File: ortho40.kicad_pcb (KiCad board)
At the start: 2 copper layers, 229 x 79.3 mm, 120 parts, among them J1 USB_mini_micro_B, K11 KEYSW, K110 KEYSW, K111 KEYSW, K112 KEYSW, K12 KEYSW, K13 KEYSW, K14 KEYSW, K15 KEYSW, K16 KEYSW, K17 KEYSW, K18 KEYSW, K19 KEYSW, K21 KEYSW, K210 KEYSW, K211 KEYSW, K212 KEYSW, K22 KEYSW, K23 KEYSW, K24 KEYSW, K25 KEYSW, K26 KEYSW, K27 KEYSW, K28 KEYSW, K29 KEYSW, K2U1 KEYSW, K2U2 KEYSW, K2U3 KEYSW, K31 KEYSW, K310 KEYSW, K311 KEYSW, K312 KEYSW, K32 KEYSW, K33 KEYSW, K34 KEYSW, K35 KEYSW, K36 KEYSW, K37 KEYSW, K38 KEYSW, K39 KEYSW, K41 KEYSW, K410 KEYSW, K411 KEYSW, K412 KEYSW, K42 KEYSW, K43 KEYSW, K44 KEYSW, K45 KEYSW, K46 KEYSW, K47 KEYSW, K48 KEYSW, K49 KEYSW, SW1 SW_PUSH, U1 ATMEGA32U4, X1 XTAL

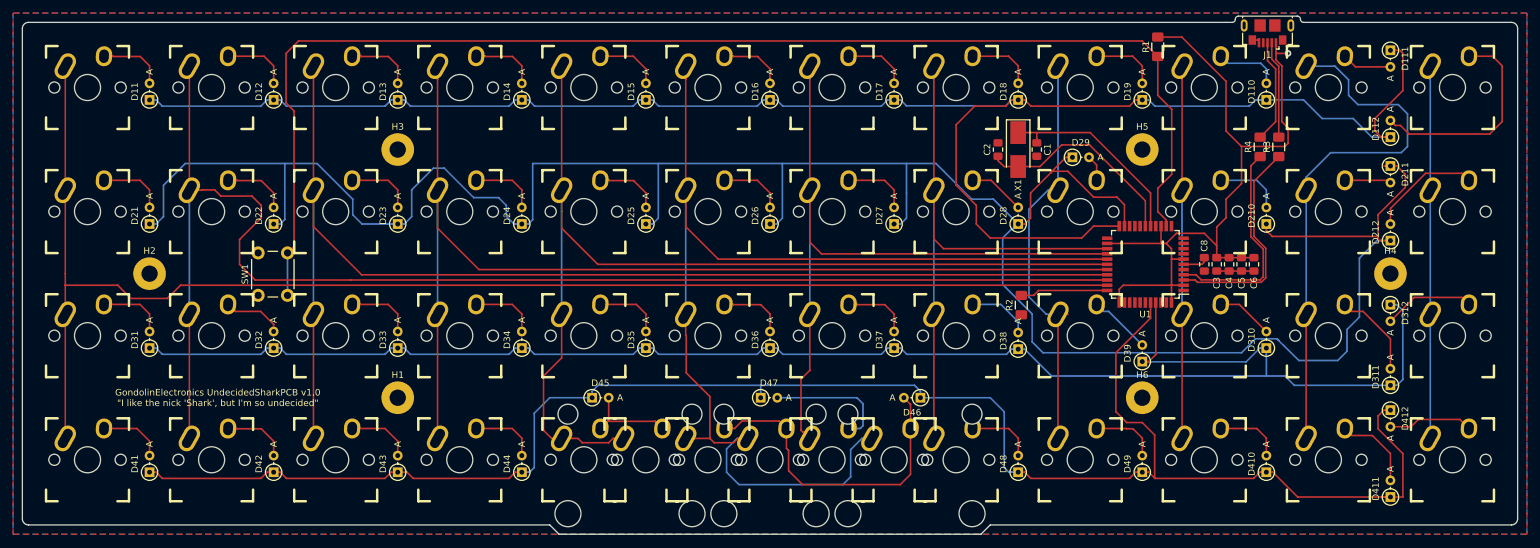
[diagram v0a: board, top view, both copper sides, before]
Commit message: Changed board size for Planck case compatibility
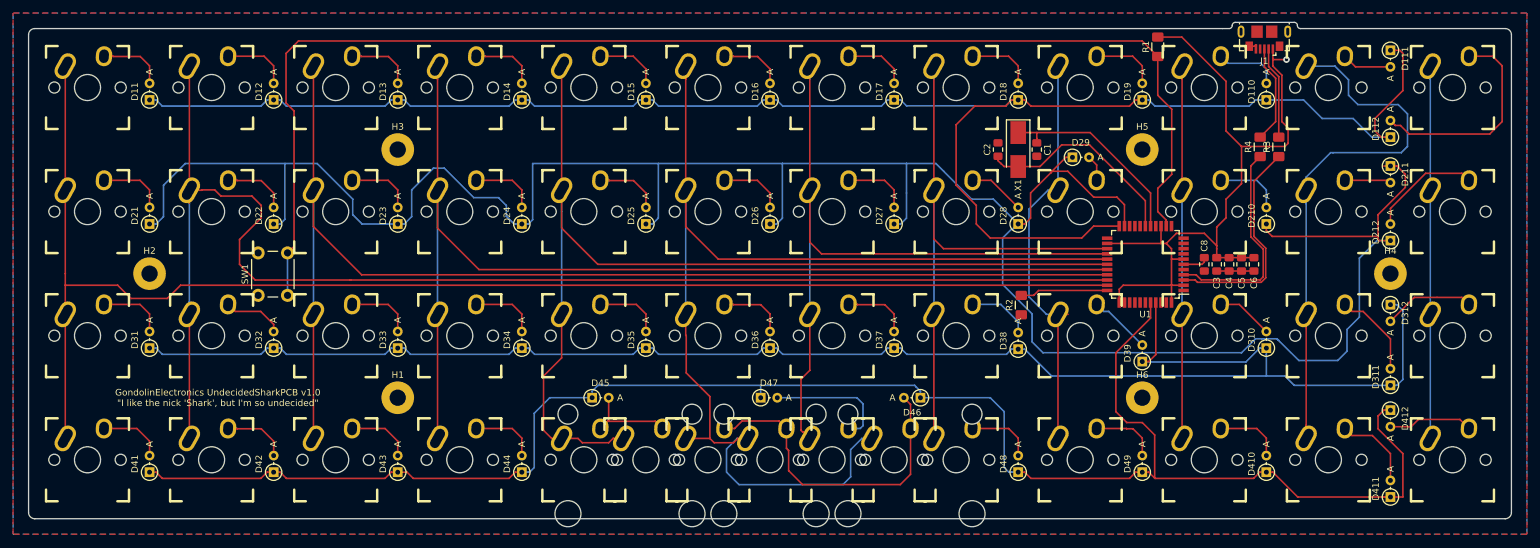
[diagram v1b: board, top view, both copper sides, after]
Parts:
- moved J1 1.06 mm to (223.9, 66.8)
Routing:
- net /D-: track 14.9 -> 14.1 mm
- net /D+: track 16.0 -> 15.2 mm
- net VCC: track 118.1 -> 117.3 mm
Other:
- board size 229 x 79.3 mm -> 227.1 x 76 mm
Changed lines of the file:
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@@
   (general
     (thickness 1.6)
-    (drawings 22)
-    (tracks 723)
+    (drawings 18)
+    (tracks 722)
     (zones 0)
     (modules 120)
@@
     (0 F.Cu signal)
     (31 B.Cu signal)
-    (32 B.Adhes user)
-    (33 F.Adhes user)
-    (34 B.Paste user)
-    (35 F.Paste user)
-    (36 B.SilkS user)
-    (37 F.SilkS user)
-    (38 B.Mask user)
-    (39 F.Mask user)
+    (32 B.Adhes user hide)
+    (33 F.Adhes user hide)
+    (34 B.Paste user hide)
+    (35 F.Paste user hide)
+    (36 B.SilkS user hide)
+    (37 F.SilkS user hide)
+    (38 B.Mask user hide)
+    (39 F.Mask user hide)
     (40 Dwgs.User user hide)
-    (41 Cmts.User user)
-    (42 Eco1.User user)
-    (43 Eco2.User user)
+    (41 Cmts.User user hide)
+    (42 Eco1.User user hide)
+    (43 Eco2.User user hide)
     (44 Edge.Cuts user)
     (45 Margin user hide)
@@
   )
   (module Connector_USB:USB_Micro-B_GCT_USB3076-30-A (layer F.Cu)
-    (at 224.375 65.8 180)
+    (at 223.9 66.75 180)
     (descr "GCT Micro USB https://gct.co/files/drawings/usb3076.pdf")
     (tags "Micro-USB SMD Typ-B GCT")
@@
     (arrow2b (pts (xy 33.725 149.625) (xy 34.851504 149.038579)))
   )
-  (gr_line (start 181.925 141.075) (end 261.725 141.075) (layer Edge.Cuts) (width 0.15))
-  (gr_line (start 180.5 142.5) (end 181.925 141.075) (layer Edge.Cuts) (width 0.15))
-  (gr_line (start 115.9 142.5) (end 180.5 142.5) (layer Edge.Cuts) (width 0.15))
-  (gr_line (start 114.475 141.075) (end 115.9 142.5) (layer Edge.Cuts) (width 0.15))
-  (gr_line (start 34.675 141.075) (end 114.475 141.075) (layer Edge.Cuts) (width 0.15))
+  (gr_line (start 35.625 140.125) (end 260.775 140.125) (layer Edge.Cuts) (width 0.15))
   (gr_text "GondolinElectronics UndecidedSharkPCB v1.0\n\"I like the nick 'Shark', but I'm so undecided\"" (at 63.65 121.6) (layer F.SilkS)
     (effects (font (size 1 1) (thickness 0.25)))
   )
-  (gr_line (start 218.975 64.125) (end 218.025 64.125) (layer Edge.Cuts) (width 0.15))
-  (gr_line (start 228.95 63.175) (end 219.925 63.175) (layer Edge.Cuts) (width 0.15))
-  (gr_arc (start 228.95 63.65) (end 229.425 63.65) (angle -90) (layer Edge.Cuts) (width 0.15))
-  (gr_arc (start 229.9 63.65) (end 229.425 63.65) (angle -90) (layer Edge.Cuts) (width 0.15))
-  (gr_arc (start 218.975 63.65) (end 218.975 64.125) (angle -90) (layer Edge.Cuts) (width 0.15))
-  (gr_arc (start 219.925 63.65) (end 219.925 63.175) (angle -90) (layer Edge.Cuts) (width 0.15))
-  (gr_line (start 229.9 64.125) (end 261.725 64.125) (layer Edge.Cuts) (width 0.15))
-  (gr_line (start 34.675 64.125) (end 218.025 64.125) (layer Edge.Cuts) (width 0.15))
-  (gr_arc (start 34.675 65.075) (end 34.675 64.125) (angle -90) (layer Edge.Cuts) (width 0.15))
-  (gr_line (start 33.725 140.125) (end 33.725 65.075) (layer Edge.Cuts) (width 0.15))
-  (gr_arc (start 34.675 140.125) (end 33.725 140.125) (angle -90) (layer Edge.Cuts) (width 0.15))
-  (gr_arc (start 261.725 140.125) (end 261.725 141.075) (angle -90) (layer Edge.Cuts) (width 0.15))
-  (gr_line (start 262.675 65.075) (end 262.675 140.125) (layer Edge.Cuts) (width 0.15))
-  (gr_arc (start 261.725 65.075) (end 262.675 65.075) (angle -90) (layer Edge.Cuts) (width 0.15))
+  (gr_line (start 218.5 65.075) (end 217.55 65.075) (layer Edge.Cuts) (width 0.15))
+  (gr_line (start 228.475 64.125) (end 219.45 64.125) (layer Edge.Cuts) (width 0.15))
+  (gr_arc (start 228.475 64.6) (end 228.95 64.6) (angle -90) (layer Edge.Cuts) (width 0.15))
+  (gr_arc (start 229.425 64.6) (end 228.95 64.6) (angle -90) (layer Edge.Cuts) (width 0.15))
+  (gr_arc (start 218.5 64.6) (end 218.5 65.075) (angle -90) (layer Edge.Cuts) (width 0.15))
+  (gr_arc (start 219.45 64.6) (end 219.45 64.125) (angle -90) (layer Edge.Cuts) (width 0.15))
+  (gr_line (start 229.425 65.075) (end 260.775 65.075) (layer Edge.Cuts) (width 0.15))
+  (gr_line (start 35.625 65.075) (end 217.55 65.075) (layer Edge.Cuts) (width 0.15))
+  (gr_arc (start 35.625 66.025) (end 35.625 65.075) (angle -90) (layer Edge.Cuts) (width 0.15))
+  (gr_line (start 34.675 139.175) (end 34.675 66.025) (layer Edge.Cuts) (width 0.15))
+  (gr_arc (start 35.625 139.175) (end 34.675 139.175) (angle -90) (layer Edge.Cuts) (width 0.15))
+  (gr_arc (start 260.775 139.175) (end 260.775 140.125) (angle -90) (layer Edge.Cuts) (width 0.15))
+  (gr_line (start 261.725 66.025) (end 261.725 139.175) (layer Edge.Cuts) (width 0.15))
+  (gr_arc (start 260.775 66.025) (end 261.725 66.025) (angle -90) (layer Edge.Cuts) (width 0.15))
   (segment (start 189.05 82.575001) (end 189.05 81.900001) (width 0.25) (layer F.Cu) (net 1) (status 10))
   (segment (start 188.149998 80.999999) (end 188.1 80.999999) (width 0.25) (layer F.Cu) (net 1))
@@
   (segment (start 216.6 102.2) (end 222.225 102.2) (width 0.25) (layer F.Cu) (net 2) (status 30))
   (segment (start 222.225 102.2) (end 222.3 102.2) (width 0.25) (layer F.Cu) (net 2) (status 30))
-  (segment (start 223.075 66.635) (end 222.88 66.83) (width 0.25) (layer F.Cu) (net 2) (status 30))
-  (segment (start 222.88 66.83) (end 222.055 66.83) (width 0.25) (layer F.Cu) (net 2) (status 30))
-  (segment (start 223.075 67.25) (end 223.075 66.635) (width 0.25) (layer F.Cu) (net 2) (status 30))
+  (segment (start 222.6 67.585) (end 222.405 67.78) (width 0.25) (layer F.Cu) (net 2) (status 30))
+  (segment (start 222.405 67.78) (end 221.58 67.78) (width 0.25) (layer F.Cu) (net 2) (status 30))
+  (segment (start 222.6 68.2) (end 222.6 67.585) (width 0.25) (layer F.Cu) (net 2) (status 30))
   (segment (start 183.1125 85.299999) (end 183.550001 85.7375) (width 0.25) (layer F.Cu) (net 3))
   (segment (start 183.1125 84.624999) (end 183.1125 85.299999) (width 0.25) (layer F.Cu) (net 3) (status 10))
@@
   (segment (start 218.025 91.2) (end 220.4 88.825) (width 0.25) (layer F.Cu) (net 4))
   (segment (start 220.4 83.125) (end 220.4 88.825) (width 0.25) (layer F.Cu) (net 4))
+  (segment (start 225.2 69.825) (end 227.05 69.825) (width 0.25) (layer F.Cu) (net 4))
+  (segment (start 225.2 68.2) (end 225.2 69.825) (width 0.25) (layer F.Cu) (net 4) (status 10))
+  (via (at 227.2875 69.825) (size 1) (drill 0.5) (layers F.Cu B.Cu) (net 4))
+  (segment (start 225.2 70.825) (end 226.575 72.2) (width 0.25) (layer F.Cu) (net 4))
   (segment (start 227.05 83.125) (end 220.4 83.125) (width 0.25) (layer F.Cu) (net 4))
-  (segment (start 225.675 69.875) (end 226.575 70.775) (width 0.25) (layer F.Cu) (net 4))
   (segment (start 227.525 80.275) (end 227.525 82.65) (width 0.25) (layer F.Cu) (net 4))
-  (segment (start 226.575 79.325) (end 227.525 80.275) (width 0.25) (layer F.Cu) (net 4))
-  (segment (start 226.575 70.775) (end 226.575 79.325) (width 0.25) (layer F.Cu) (net 4))
+  (segment (start 225.2 69.825) (end 225.2 70.825) (width 0.25) (layer F.Cu) (net 4))
   (segment (start 227.525 82.65) (end 227.05 83.125) (width 0.25) (layer F.Cu) (net 4))
-  (segment (start 225.675 68.875) (end 227.525 68.875) (width 0.25) (layer F.Cu) (net 4))
-  (segment (start 225.675 68.875) (end 225.675 69.875) (width 0.25) (layer F.Cu) (net 4))
-  (segment (start 225.675 67.25) (end 225.675 68.875) (width 0.25) (layer F.Cu) (net 4) (status 10))
-  (via (at 227.525 68.875) (size 1) (drill 0.5) (layers F.Cu B.Cu) (net 4))
+  (segment (start 226.575 72.2) (end 226.575 79.325) (width 0.25) (layer F.Cu) (net 4))
+  (segment (start 226.575 79.325) (end 227.525 80.275) (width 0.25) (layer F.Cu) (net 4))
   (segment (start 211.525 101.175) (end 214.35 101.175) (width 0.25) (layer F.Cu) (net 5) (status 10))
   (segment (start 214.7 100.825) (end 214.7 100.15) (width 0.25) (layer F.Cu) (net 5) (status 20))
@@
   (segment (start 243.2 126.04) (end 246.36 126.04) (width 0.25) (layer F.Cu) (net 55) (status 10))
   (segment (start 246.36 126.04) (end 247.475 124.925) (width 0.25) (layer F.Cu) (net 55))
-  (segment (start 226.1 71.725) (end 226.1 81.7) (width 0.25) (layer F.Cu) (net 56) (status 20))
-  (segment (start 226.1 70.837414) (end 226.1 71.725) (width 0.25) (layer F.Cu) (net 56))
-  (segment (start 225.025 67.25) (end 225.025001 69.762415) (width 0.25) (layer F.Cu) (net 56) (status 10))
-  (segment (start 225.025001 69.762415) (end 226.1 70.837414) (width 0.25) (layer F.Cu) (net 56))
-  (segment (start 225.625 79.325) (end 223.25 81.7) (width 0.25) (layer F.Cu) (net 58) (status 20))
-  (segment (start 225.625 71.25) (end 225.625 79.325) (width 0.25) (layer F.Cu) (net 58))
-  (segment (start 224.375 70) (end 225.625 71.25) (width 0.25) (layer F.Cu) (net 58))
-  (segment (start 224.375 67.25) (end 224.375 70) (width 0.25) (layer F.Cu) (net 58) (status 10))
+  (segment (start 226.1 72.4375) (end 226.1 81.7) (width 0.25) (layer F.Cu) (net 56))
+  (segment (start 224.55 68.2) (end 224.550001 70.887501) (width 0.25) (layer F.Cu) (net 56))
+  (segment (start 224.550001 70.887501) (end 226.1 72.4375) (width 0.25) (layer F.Cu) (net 56))
+  (segment (start 225.625 79.325) (end 223.25 81.7) (width 0.25) (layer F.Cu) (net 58))
+  (segment (start 225.625 72.675) (end 225.625 79.325) (width 0.25) (layer F.Cu) (net 58))
+  (segment (start 223.9 68.2) (end 223.9 70.95) (width 0.25) (layer F.Cu) (net 58))
+  (segment (start 223.9 70.95) (end 225.625 72.675) (width 0.25) (layer F.Cu) (net 58))
   (segment (start 40.295 70.83) (end 40.295 89.83) (width 0.25) (layer F.Cu) (net 59) (status 30))
   (segment (start 40.295 108.83) (end 40.295 127.83) (width 0.25) (layer F.Cu) (net 59) (status 30))
